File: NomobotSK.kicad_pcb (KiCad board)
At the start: 2 copper layers, 106.8 x 107.5 mm, 74 parts, among them J1 Conn_01x12_Pin, J2 Conn_01x03_Socket, J3 Conn_01x03_Socket, J4 Conn_01x03_Socket, J5 Conn_01x12_Pin, J6 Conn_01x12_Pin, M1 Motor_DC, M2 Motor_DC, SW1 SW_DIP_x01, SW2 SW_Push, SW3 SW_Push, SW4 SW_Push, SW5 SW_DIP_x10, SW6 SW_DIP_x04, U1 L293D, U2 TP4056 Module, U3 TCRT5000, U4 TCRT5000, U5 HC-SR04, U6 AMS1117-3.3, U7 LM393D

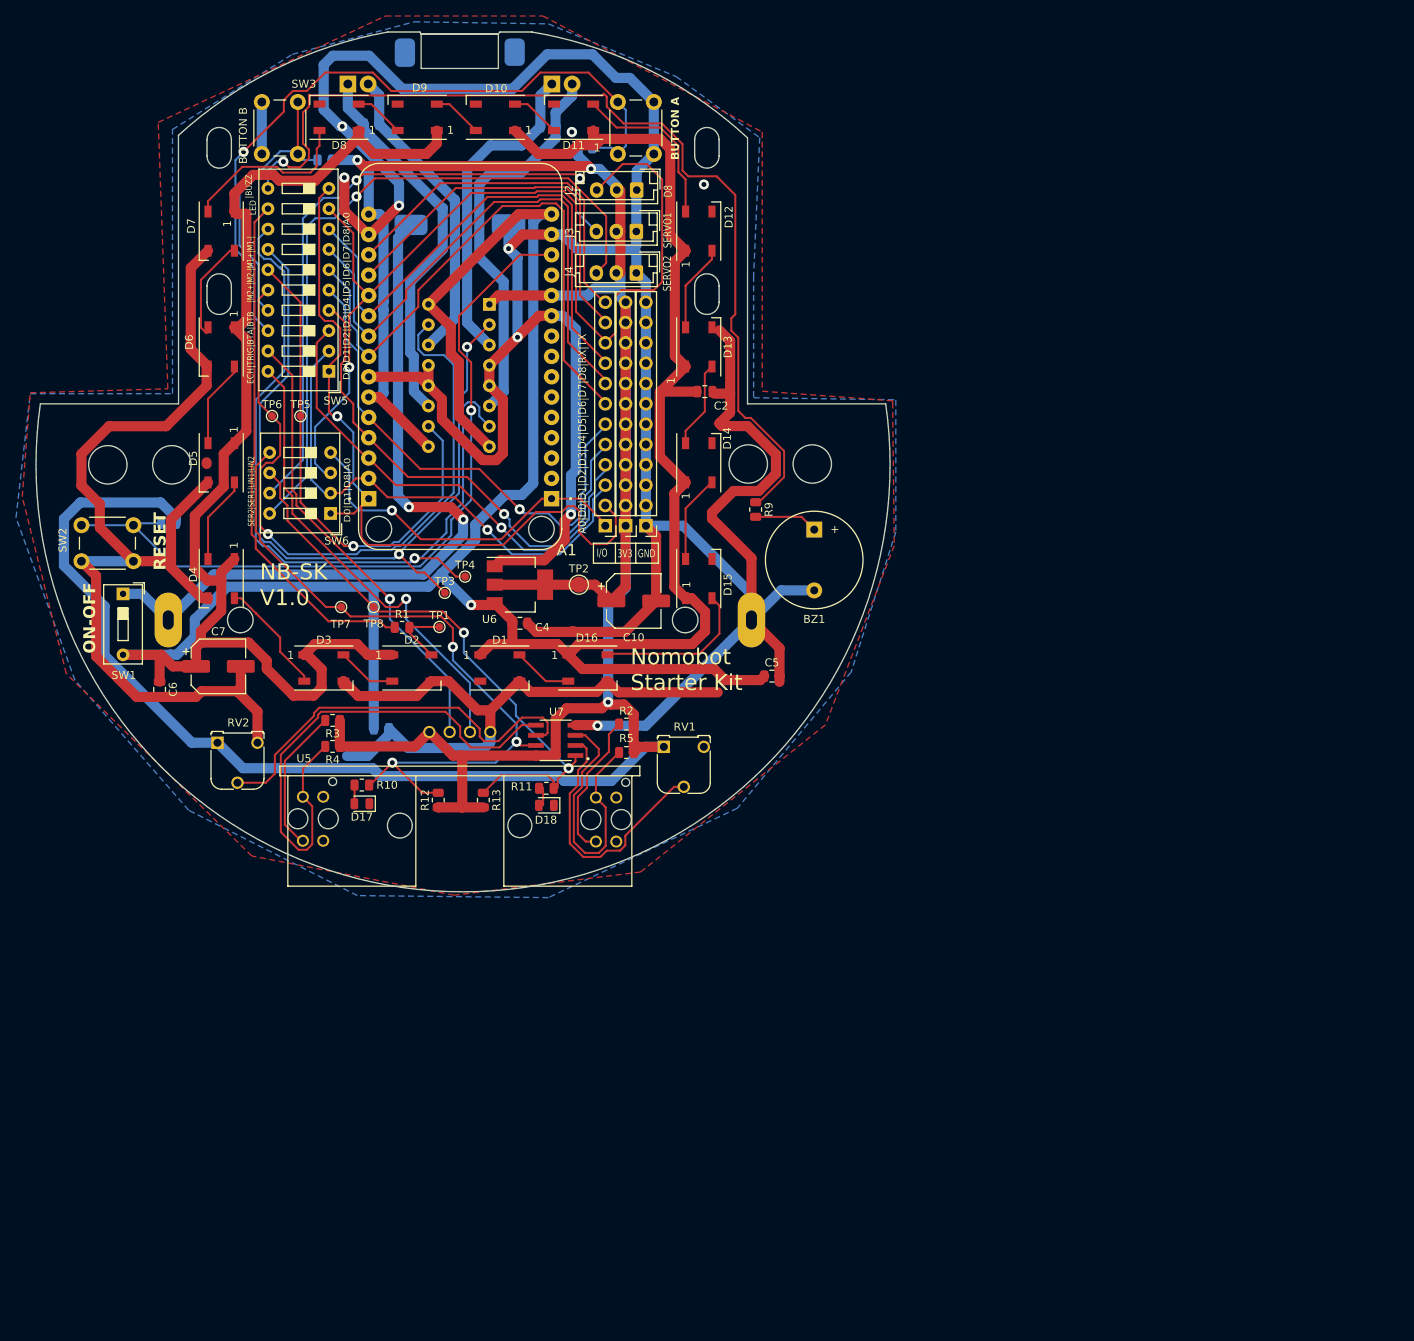
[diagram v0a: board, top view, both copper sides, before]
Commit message: routing done
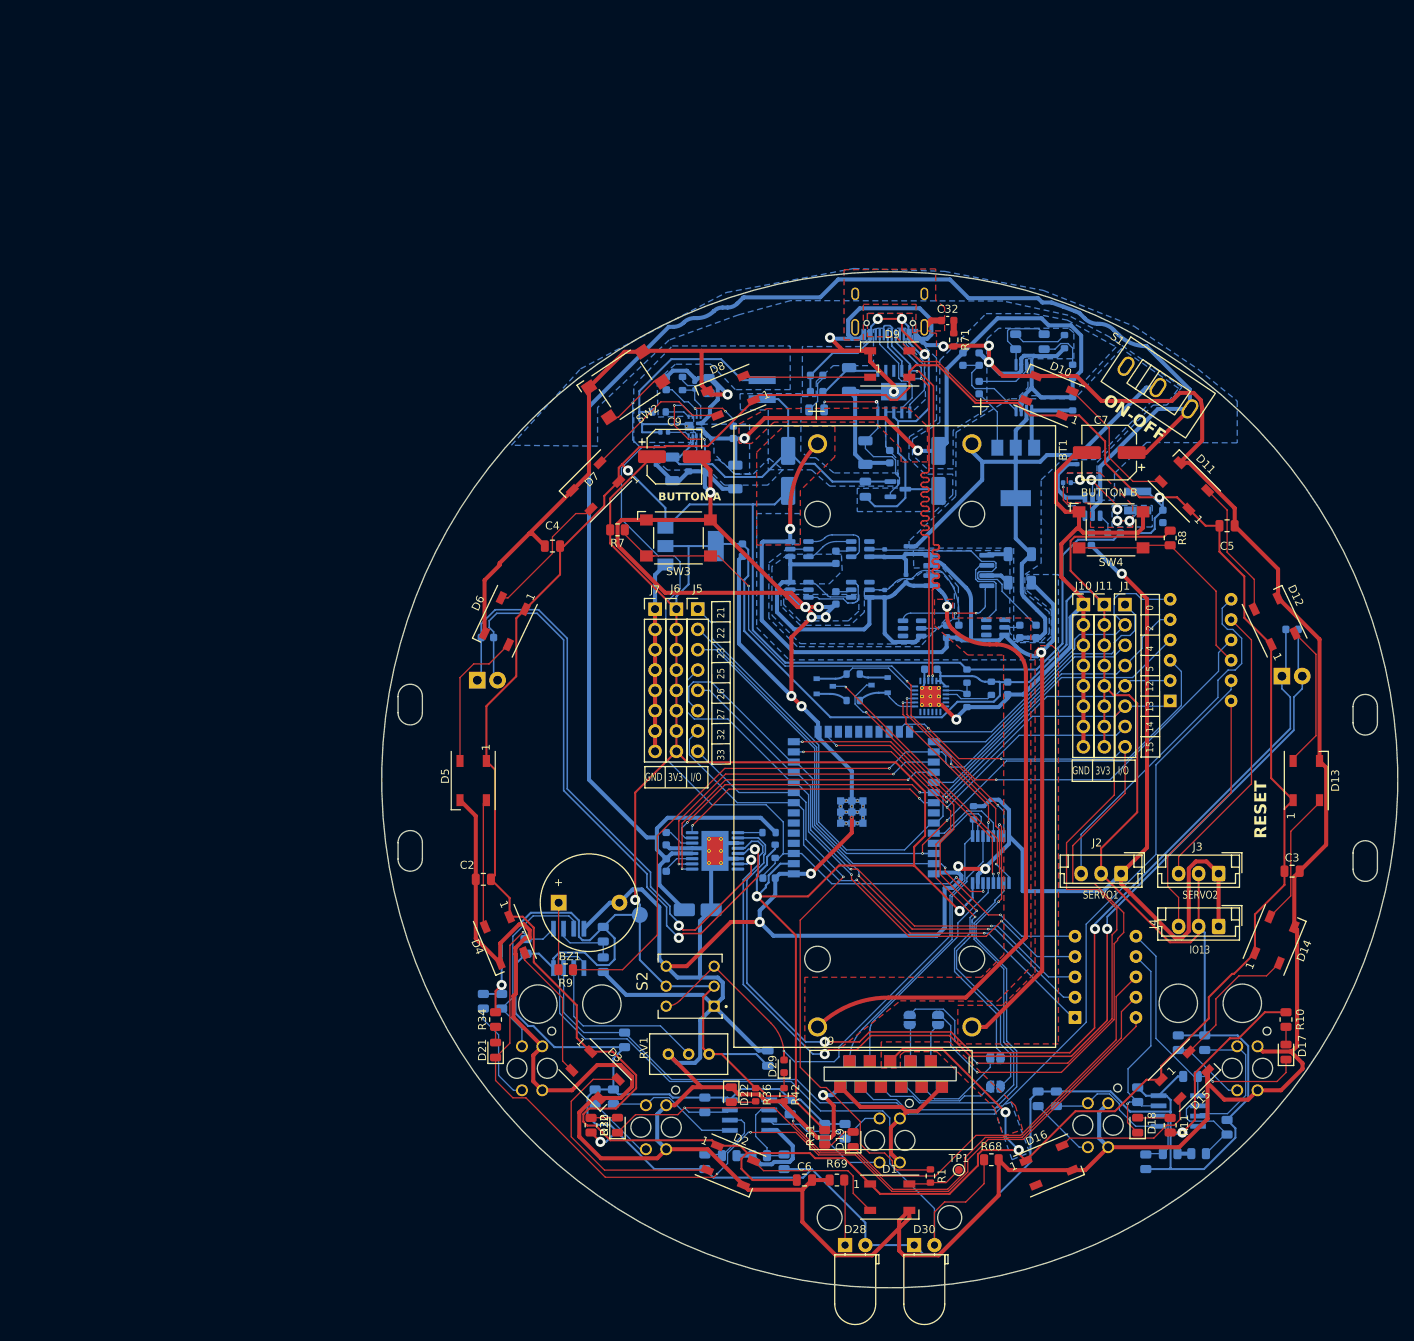
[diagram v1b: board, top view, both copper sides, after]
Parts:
- removed A1: NodeMCU V2 Amica, NodeMCU V2 AMICA:NodeMCU V2 Amica
- removed RV2: Trimpot_10K, Potentiometer_THT:Potentiometer_Runtron_RM-065_Vertical
- removed SW1: SW_DIP_x01, Button_Switch_THT:SW_DIP_SPSTx01_Slide_9.78x4.72mm_W7.62mm_P2.54mm
- removed TP3, TP4, TP5, TP6, TP7, TP8: TestPoint, TestPoint:TestPoint_Pad_D1.0mm
- added C11: 100nF, Capacitor_SMD:C_0603_1608Metric, B.Cu at (187.3, 112.3)
- added C12: 22uF/20V, Capacitor_SMD:C_0805_2012Metric, B.Cu at (190.5, 175.8)
- added C13: 4.7uF/6.3V, Capacitor_SMD:C_0603_1608Metric, B.Cu at (210.9, 127.2)
- added C14: 100nF/50V, Capacitor_SMD:C_0603_1608Metric, B.Cu at (220.5, 129.5)
- added C15: 100nF, Capacitor_SMD:C_0402_1005Metric, B.Cu at (177.5, 97.5)
- added C16: 47uF, Capacitor_SMD:C_1206_3216Metric, B.Cu at (186.4, 103.1)
- added C17: 47uF, Capacitor_SMD:C_1206_3216Metric, B.Cu at (178.6, 102.1)
- added C18: 100nF, Capacitor_SMD:C_0402_1005Metric, B.Cu at (176.5, 101.1)
- added C19: 10uF, Capacitor_SMD:C_0603_1608Metric, B.Cu at (182.6, 101.6)
- added C20: 470pF, Capacitor_SMD:C_0805_2012Metric, B.Cu at (183.1, 91.7)
- added C21: 24pF, Capacitor_SMD:C_0402_1005Metric, B.Cu at (181.4, 91.7)
- added C22: 100nF, Capacitor_SMD:C_0402_1005Metric, B.Cu at (207.8, 112.3)
- added C23: 100nF, Capacitor_SMD:C_0402_1005Metric, B.Cu at (207.8, 115.8)
- added C24: 100nF, Capacitor_SMD:C_0402_1005Metric, B.Cu at (205.1, 112.6)
- added C25: 100nF, Capacitor_SMD:C_0402_1005Metric, B.Cu at (205.1, 117.7)
- added C26: 1uF, Capacitor_SMD:C_1206_3216Metric, B.Cu at (200.7, 90.9)
- added C27: 1uF, Capacitor_SMD:C_1206_3216Metric, B.Cu at (202.7, 100.1)
- added C28: 100nF, Capacitor_SMD:C_0402_1005Metric, B.Cu at (229.2, 101.0)
- added C29: 10nF, Capacitor_SMD:C_0603_1608Metric, B.Cu at (177.8, 151.6)
- added C30: 100nF, Capacitor_SMD:C_0603_1608Metric, B.Cu at (256.0, 122.2)
- added C31: 100nF, Capacitor_SMD:C_0603_1608Metric, B.Cu at (155.4, 123.2)
- added C32: 100nF, Capacitor_SMD:C_0603_1608Metric, F.Cu at (213.0, 83.6)
- added C33: 100nF, Capacitor_SMD:C_0402_1005Metric, B.Cu at (227.9, 103.8)
- added C34: 22uF, Capacitor_SMD:C_0603_1608Metric, B.Cu at (239.9, 108.1)
- added C9: 22uF, Capacitor_SMD:CP_Elec_6.3x5.3, F.Cu at (178.8, 100.6)
- added D19: LED_Green, LED_SMD:LED_0805_2012Metric, F.Cu at (201.2, 185.9)
- added D20: LED_Green, LED_SMD:LED_0805_2012Metric, F.Cu at (171.7, 184.2)
- added D21: LED_Green, LED_SMD:LED_0805_2012Metric, F.Cu at (156.5, 174.8)
- added D22: LED_Blue, LED_SMD:LED_0805_2012Metric, F.Cu at (185.9, 180.3)
- added D23: LED_Red, LED_SMD:LED_0805_2012Metric, B.Cu at (221.5, 86.2)
- added D24: LED_Blue, LED_SMD:LED_0805_2012Metric, B.Cu at (196.6, 94.7)
- added D25: SS34, Diode_SMD:D_SMA_Handsoldering, B.Cu at (211.8, 102.4)
- added D26: SS34, Diode_SMD:D_SMA_Handsoldering, B.Cu at (193.0, 102.4)
- added D27: LED_Green, LED_SMD:LED_0805_2012Metric, B.Cu at (225.0, 86.2)
- added D28: IR_LED, LED_THT:LED_D5.0mm_Horizontal_O1.27mm_Z3.0mm_IRBlack, F.Cu at (200.2, 199.1)
- added D29: LED_RED, LED_SMD:LED_0603_1608Metric, F.Cu at (192.5, 176.8)
- added D30: IR_Photodiode, LED_THT:LED_D5.0mm_Horizontal_O1.27mm_Z3.0mm_Clear, F.Cu at (208.8, 199.1)
- added IC1: TS3A5018PW, TS3A5018PW:SOP65P640X120-16N, B.Cu at (218.4, 150.9)
- added J10: Conn_01x08_Pin, Connector_PinHeader_2.54mm:PinHeader_1x08_P2.54mm_Vertical, F.Cu at (229.9, 119.1)
- added J11: Conn_01x08_Pin, Connector_PinHeader_2.54mm:PinHeader_1x08_P2.54mm_Vertical, F.Cu at (232.6, 119.1)
- added J7: Conn_01x08_Pin, Connector_PinHeader_2.54mm:PinHeader_1x08_P2.54mm_Vertical, F.Cu at (176.4, 119.6)
- added J8: USB_C_Receptacle_USB2.0, Connector_USB:USB_C_Receptacle_HRO_TYPE-C-31-M-12, B.Cu at (205.7, 81.3)
- added J9: Conn_ESPCAM_Shield, Connector_Custom:Conn_ESPCAM_Shield-Female, F.Cu at (205.8, 178.7)
- added JP1: SolderJumper_2_Open, Jumper:SolderJumper-2_P1.3mm_Open_RoundedPad1.0x1.5mm, B.Cu at (218.9, 175.8)
- added JP2: SolderJumper_2_Open, Jumper:SolderJumper-2_P1.3mm_Open_RoundedPad1.0x1.5mm, B.Cu at (208.2, 171.0)
- added JP3: SolderJumper_2_Open, Jumper:SolderJumper-2_P1.3mm_Open_RoundedPad1.0x1.5mm, B.Cu at (211.8, 171.0)
- added JP4: SolderJumper_2_Open, Jumper:SolderJumper-2_P1.3mm_Open_RoundedPad1.0x1.5mm, B.Cu at (218.9, 179.3)
- added L1: XAL4020-102MEB_1uH, Inductor_SMD:L_Coilcraft_XAL4020-XXX, B.Cu at (189.8, 92.2)
- added L2: XAL4030-332MEB_3.3uH, Inductor_SMD:L_Coilcraft_XAL4030-XXX, B.Cu at (236.7, 106.1)
- added Q1: SS8050-G, SS8050-G:TRANS_SS8050-G, B.Cu at (204.5, 129.1)
- added Q2: SS8050-G, SS8050-G:TRANS_SS8050-G, B.Cu at (197.6, 129.3)
- added Q3: DMG9926UDM, Package_TO_SOT_SMD:SOT-23-6, B.Cu at (194.4, 112.1)
- added Q4: DMG9926UDM, Package_TO_SOT_SMD:SOT-23-6, B.Cu at (194.4, 117.2)
- added Q5: DMG9926USD-13, Package_SO:SO-8_5.3x6.2mm_P1.27mm, B.Cu at (214.4, 114.8)
- added Q6: AO3400A, Package_TO_SOT_SMD:SOT-23, B.Cu at (206.8, 104.6)
- added Q7: FZT788BTA, Package_TO_SOT_SMD:SOT-223-3_TabPin2, B.Cu at (221.5, 102.6)
- added R14: 220R, Resistor_SMD:R_0805_2012Metric, B.Cu at (197.6, 184.9)
- added R15: 220R, Resistor_SMD:R_0805_2012Metric, B.Cu at (168.9, 180.6)
- added R16: 10K, Resistor_SMD:R_0805_2012Metric, B.Cu at (200.2, 184.9)
- added R17: 10K, Resistor_SMD:R_0805_2012Metric, B.Cu at (171.2, 180.6)
- added R18: 220R, Resistor_SMD:R_0805_2012Metric, B.Cu at (154.9, 168.7)
- added R19: 10K, Resistor_SMD:R_0805_2012Metric, B.Cu at (157.2, 168.7)
- added R20: 10K, Resistor_SMD:R_0805_2012Metric, B.Cu at (240.8, 187.7)
- added R21: 10K, Resistor_SMD:R_0805_2012Metric, B.Cu at (237.7, 188.7)
- added R22: 10K, Resistor_SMD:R_0805_2012Metric, B.Cu at (247.9, 184.4)
- added R23: 10K, Resistor_SMD:R_0805_2012Metric, B.Cu at (244.3, 187.7)
- added R24: 10K, Resistor_SMD:R_0805_2012Metric, B.Cu at (192.5, 188.7)
- added R25: 10K, Resistor_SMD:R_0805_2012Metric, B.Cu at (182.6, 188.7)
- added R26: 10K, Resistor_SMD:R_0805_2012Metric, B.Cu at (185.7, 188.0)
- added R27: 10K, Resistor_SMD:R_0805_2012Metric, B.Cu at (189.5, 188.0)
- added R28: 10K, Resistor_SMD:R_0805_2012Metric, B.Cu at (182.6, 181.6)
- added R29: 10K, Resistor_SMD:R_0805_2012Metric, B.Cu at (193.3, 181.9)
- added R30: 10K, Resistor_SMD:R_0805_2012Metric, B.Cu at (169.9, 160.3)
- added R31: 470R, Resistor_SMD:R_0805_2012Metric, F.Cu at (197.6, 185.7)
- added R32: 470R, Resistor_SMD:R_0805_2012Metric, F.Cu at (168.4, 184.2)
- added R33: 10K, Resistor_SMD:R_0805_2012Metric, B.Cu at (169.9, 164.1)
- added R34: 470R, Resistor_SMD:R_0805_2012Metric, F.Cu at (156.5, 170.9)
- added R35: 10K, Resistor_SMD:R_0805_2012Metric, B.Cu at (160.3, 161.8)
- added R36: 220R, Resistor_SMD:R_0603_1608Metric, F.Cu at (189.0, 180.3)
- added R37: 28.7K, Resistor_SMD:R_0603_1608Metric, B.Cu at (179.8, 91.4)
- added R38: 10K, Resistor_SMD:R_0603_1608Metric, B.Cu at (201.2, 127.8)
- added R39: 10K, Resistor_SMD:R_0603_1608Metric, B.Cu at (201.2, 131.1)
- added R40: 10K, Resistor_SMD:R_0603_1608Metric, B.Cu at (218.4, 129.5)
- added R41: 10K, Resistor_SMD:R_0603_1608Metric, B.Cu at (216.2, 145.1)
- added R42: 330R, Resistor_SMD:R_0603_1608Metric, F.Cu at (192.5, 180.3)
- added R43: 22.1K, Resistor_SMD:R_0603_1608Metric, B.Cu at (215.4, 128.0)
- added R44: 47.5K, Resistor_SMD:R_0603_1608Metric, B.Cu at (215.4, 131.1)
- added R45: 649K, Capacitor_SMD:C_0603_1608Metric, B.Cu at (186.2, 97.5)
- added R46: 101K, Capacitor_SMD:C_0603_1608Metric, B.Cu at (177.8, 91.4)
- added R47: 100K, Resistor_SMD:R_0603_1608Metric, B.Cu at (176.9, 95.0)
- added R48: 107K, Resistor_SMD:R_0603_1608Metric, B.Cu at (180.6, 101.6)
- added R49: 1K, Resistor_SMD:R_1206_3216Metric, B.Cu at (222.0, 112.8)
- added R50: 1K, Resistor_SMD:R_1206_3216Metric, B.Cu at (222.0, 116.3)
- added R51: 100R, Capacitor_SMD:C_0603_1608Metric, B.Cu at (222.0, 122.4)
- added R52: 100R, Capacitor_SMD:C_0603_1608Metric, B.Cu at (212.9, 122.4)
- added R53: 100R, Capacitor_SMD:C_0603_1608Metric, B.Cu at (224.0, 122.4)
- added R54: 1K, Capacitor_SMD:C_0603_1608Metric, B.Cu at (199.0, 113.2)
- added R55: 1K, Capacitor_SMD:C_0603_1608Metric, B.Cu at (199.0, 118.2)
- added R56: 100R, Capacitor_SMD:C_0603_1608Metric, B.Cu at (214.4, 122.4)
- added R57: 6.8K, Capacitor_SMD:C_0603_1608Metric, B.Cu at (205.7, 100.6)
- added R58: 1K, Capacitor_SMD:C_0603_1608Metric, B.Cu at (196.6, 92.5)
- added R59: 1K, Capacitor_SMD:C_0603_1608Metric, B.Cu at (196.6, 90.4)
- added R60: 0R, Capacitor_SMD:C_0805_2012Metric, B.Cu at (202.7, 104.6)
- added R61: 1K, Capacitor_SMD:C_0603_1608Metric, B.Cu at (216.9, 91.9)
- added R62: 280R, Resistor_SMD:R_0603_1608Metric, B.Cu at (227.6, 86.2)
- added R63: 280R, Resistor_SMD:R_0603_1608Metric, B.Cu at (228.6, 89.9)
- added R64: 0.2R, Resistor_SMD:R_0603_1608Metric, B.Cu at (228.6, 94.0)
- added R65: 1K, Capacitor_SMD:C_0603_1608Metric, B.Cu at (214.9, 88.4)
- added R66: 1K, Capacitor_SMD:C_0603_1608Metric, B.Cu at (216.9, 88.4)
- added R67: 47K, Resistor_SMD:R_0603_1608Metric, B.Cu at (190.7, 147.6)
- added R68: 10K, Resistor_SMD:R_0805_2012Metric, F.Cu at (218.4, 188.5)
- added R69: 220R, Resistor_SMD:R_0805_2012Metric, F.Cu at (199.1, 191.0)
- added R70: 10K, Resistor_SMD:R_0805_2012Metric, B.Cu at (172.6, 173.5)
- added R71: 220R, Resistor_SMD:R_0603_1608Metric, F.Cu at (213.7, 86.0)
- added R72: 10K, Capacitor_SMD:C_0603_1608Metric, B.Cu at (230.9, 110.9)
- added R73: 56.2K, Capacitor_SMD:C_0603_1608Metric, B.Cu at (233.8, 110.1)
- added S1: SW_SS12D10, Switch Custom:SW_SS-12D10-G5050, F.Cu at (239.3, 91.9)
- added S2: SW_DPDT_TL2285EE, Switch Custom:SW_TL2285EE, F.Cu at (180.8, 166.8)
- added U10: TCRT5000, TCRT5000:OPTO_TCRT5000, B.Cu at (161.0, 177.0)
- added U11: LM393D, LM393D:SOIC127P599X175-8N, B.Cu at (188.2, 182.9)
- added U12: LM393D, LM393D:SOIC127P599X175-8N, B.Cu at (165.6, 162.1)
- added U13: ESP32-WROOM-32E__16MB_, ESP32-WROOM-32E:XCVR_ESP32-WROOM-32E__16MB_, B.Cu at (202.5, 147.5)
- added U14: CP2102N-Axx-xQFN24, Package_DFN_QFN:QFN-24-1EP_4x4mm_P0.5mm_EP2.6x2.6mm_ThermalVias, B.Cu at (210.8, 130.6)
- added U15: DW01A, Package_TO_SOT_SMD:SOT-23-6, B.Cu at (202.1, 112.1)
- added U16: DW01A, Package_TO_SOT_SMD:SOT-23-6, B.Cu at (202.1, 117.2)
- added U17: HY2213-BB3A, Package_TO_SOT_SMD:SOT-23-6, B.Cu at (218.9, 121.9)
- added U18: HY2213-BB3A, Package_TO_SOT_SMD:SOT-23-6, B.Cu at (208.5, 122.0)
- added U19: CH224K, CH224K:ESSOP-10, B.Cu at (206.2, 92.5)
- added U21: BQ2057WTSTR, Package_SO:TSSOP-8_4.4x3mm_P0.65mm, B.Cu at (222.5, 91.9)
- added U8: TCRT5000, TCRT5000:OPTO_TCRT5000, B.Cu at (205.7, 186.1)
- added U9: TCRT5000, TCRT5000:OPTO_TCRT5000, B.Cu at (176.5, 184.4)
- BT1: value BH-18650-PC -> BK-18650-PC4; footprint BH-18650-PC:BAT_BH-18650-PC -> BK-18650-PC4:BAT_BK-18650-PC4; moved to F.Cu
- C1: value 1u -> 10uF/16V; footprint Capacitor_SMD:C_0805_2012Metric -> Capacitor_SMD:C_Elec_4x5.4
- C10: value C_Polarized -> 100nF; footprint Capacitor_SMD:CP_Elec_6.3x5.3 -> Capacitor_SMD:C_0603_1608Metric; moved to B.Cu
- C2, C4, C5, C6: value 100n -> 100nF
- C3: value 100n -> 100nF; moved to F.Cu
- C7: value C_Polarized -> 10uF
- C8: value 1u -> 2.2uF; footprint Capacitor_SMD:C_0805_2012Metric -> Capacitor_SMD:C_0603_1608Metric
- J1, J5, J6: value Conn_01x12_Pin -> Conn_01x08_Pin; footprint Connector_PinHeader_2.54mm:PinHeader_1x12_P2.54mm_Vertical -> Connector_PinHeader_2.54mm:PinHeader_1x08_P2.54mm_Vertical
- R1, R6: footprint Resistor_SMD:R_0805_2012Metric -> Resistor_SMD:R_0603_1608Metric
- R10, R11: value 330R -> 470R
- R12, R13: value 1K -> 10K; moved to B.Cu
- R2, R3, R4, R5, TP2, U6, U7: moved to B.Cu
- R7, R8: moved to F.Cu
- RV1: value Trimpot_10K -> R_Potentiometer_10K; footprint Potentiometer_THT:Potentiometer_Runtron_RM-065_Vertical -> Potentiometer_THT:Potentiometer_Bourns_3296W_Vertical
- SW2, SW3, SW4: value SW_Push -> SW_SPST_Omron_B3FS-105xP; footprint Button_Switch_THT:SW_PUSH_6mm_H4.3mm -> Button_Switch_SMD:SW_SPST_Omron_B3FS-105xP
- SW5: value SW_DIP_x10 -> SW_DIP_x06; footprint Button_Switch_THT:SW_DIP_SPSTx10_Slide_9.78x27.58mm_W7.62mm_P2.54mm -> Button_Switch_THT:SW_DIP_SPSTx06_Slide_9.78x17.42mm_W7.62mm_P2.54mm; moved to B.Cu
- SW6: value SW_DIP_x04 -> SW_DIP_x05; footprint Button_Switch_THT:SW_DIP_SPSTx04_Slide_9.78x12.34mm_W7.62mm_P2.54mm -> Button_Switch_THT:SW_DIP_SPSTx05_Slide_9.78x14.88mm_W7.62mm_P2.54mm; moved to B.Cu
- U1: value L293D -> DRV8833PWP; footprint Package_DIP:DIP-16_W7.62mm -> Package_SO:HTSSOP-16-1EP_4.4x5mm_P0.65mm_EP3.4x5mm_Mask2.46x2.31mm_ThermalVias
- U2: value TP4056 Module -> TPS61089RNRR; footprint Modules:TP4056_Module -> TPS61089RNRR:IC_TPS61089RNRR
- U5: value HC-SR04 -> TPS563201; footprint HC-SR04:XCVR_HC-SR04 -> Package_TO_SOT_SMD:SOT-23-6; moved to B.Cu
- moved D17 119.6 mm to (255.3, 175.0), turned to 90 degrees
- moved R10 119.2 mm to (255.3, 170.9), turned to 90 degrees
- moved M1 117.5 mm to (254.8, 128.0)
- moved R8 115.7 mm to (240.8, 110.7), turned to 90 degrees
- moved C3 115.2 mm to (256.0, 152.4)
- moved C7 114.5 mm to (233.2, 100.1), turned to 180 degrees
- moved SW5 112.9 mm to (240.8, 131.1), turned to 0 degrees
- moved SW6 112.4 mm to (228.9, 170.7), turned to 0 degrees
- moved J4 109.4 mm to (246.8, 159.3)
- moved J3 108.4 mm to (246.8, 152.7)
- moved C1 106.3 mm to (181.7, 157.2)
- moved U4 105.3 mm to (231.8, 184.2)
- moved J2 104.7 mm to (234.7, 152.7)
- moved C6 101.3 mm to (195.1, 191.0), turned to 0 degrees
- moved R4 100.6 mm to (226.6, 180.8), turned to -90 degrees
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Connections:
- net SIG_L renamed /LINE SENSOR/SIG_1
- net SIG_R renamed /LINE SENSOR/SIG_2
- C1 pad 1: M2P -> /POWER/VBAT
- C1 pad 2: M2N -> GND
- C10 pad 1: 3V3 -> GND
- C10 pad 2: GND -> /MAIN MCU/EN
- C2 pad 1: VBAT+ -> /VCC
- C3 pad 1: VBAT+ -> /VCC
- C4 pad 1: VBAT+ -> /VCC
- C5 pad 1: VBAT+ -> /VCC
- C6 pad 1: VBAT+ -> /VCC
- C7 pad 1: VBAT+ -> /POWER/VBAT
- C8 pad 1: M1P -> Net-(U1-VINT)
- C8 pad 2: M1N -> GND
- D1 pad 1: VBAT+ -> /VCC
- D1 pad 2: unconnected-(D1-DOUT-Pad2) -> Net-(D1-DOUT)
- D1 pad 4: Net-(D1-DIN) -> /MAIN MCU/LED_DIN
- D10 pad 1: VBAT+ -> /VCC
- D11 pad 1: VBAT+ -> /VCC
- D12 pad 1: VBAT+ -> /VCC
- D13 pad 1: VBAT+ -> /VCC
- D14 pad 1: VBAT+ -> /VCC
- D15 pad 1: VBAT+ -> /VCC
- D16 pad 1: VBAT+ -> /VCC
- D16 pad 2: Net-(D1-DIN) -> unconnected-(D16-DOUT-Pad2)
- D17 pad 1: GND -> /LINE SENSOR/LIN_1
- D18 pad 1: GND -> /LINE SENSOR/LIN_2
- D2 pad 1: VBAT+ -> /VCC
- D2 pad 4: LED_DIN -> Net-(D1-DOUT)
- D3 pad 1: VBAT+ -> /VCC
- D4 pad 1: VBAT+ -> /VCC
- D5 pad 1: VBAT+ -> /VCC
- D6 pad 1: VBAT+ -> /VCC
- D7 pad 1: VBAT+ -> /VCC
- D8 pad 1: VBAT+ -> /VCC
- D9 pad 1: VBAT+ -> /VCC
- J1 pad 1: A0 -> /MAIN MCU/IO0
- J1 pad 2: D0 -> /MAIN MCU/IO2
- J1 pad 3: D1 -> /MAIN MCU/IO4
- J1 pad 4: D2 -> /MAIN MCU/IO5
- J1 pad 5: D3 -> /MAIN MCU/IO12
- J1 pad 6: D4 -> /MAIN MCU/IO13
- J1 pad 7: D5 -> /MAIN MCU/IO14
- J1 pad 8: D6 -> /MAIN MCU/IO15
- J2 pad 2: 3V3 -> /VDD
- J2 pad 3: D8 -> /MAIN MCU/SERVO_R
- J3 pad 2: 3V3 -> /VDD
- J3 pad 3: SERVO_R -> /MAIN MCU/SERVO_L
- J4 pad 2: 3V3 -> /VDD
- J4 pad 3: SERVO_L -> /MAIN MCU/I/O Pin
- J5 pad 1: 3V3 -> /MAIN MCU/IO21
- J5 pad 2: 3V3 -> /MAIN MCU/IO22
- J5 pad 3: 3V3 -> /MAIN MCU/IO23
- J5 pad 4: 3V3 -> /MAIN MCU/IO25
- J5 pad 5: 3V3 -> /MAIN MCU/IO26
- J5 pad 6: 3V3 -> /MAIN MCU/IO27
- J5 pad 7: 3V3 -> /MAIN MCU/IO32
- J5 pad 8: 3V3 -> /MAIN MCU/IO33
- J6 pad 1: GND -> /VDD
- J6 pad 2: GND -> /VDD
- J6 pad 3: GND -> /VDD
- J6 pad 4: GND -> /VDD
- J6 pad 5: GND -> /VDD
- J6 pad 6: GND -> /VDD
- J6 pad 7: GND -> /VDD
- J6 pad 8: GND -> /VDD
- R1 pad 1: Net-(R1-Pad1) -> /MAIN MCU/IO33
- R1 pad 2: LED_DIN -> /MAIN MCU/LED_DIN
- R10 pad 1: LIN_R -> Net-(D17-A)
- R10 pad 2: Net-(D17-A) -> /VDD
- R11 pad 1: LIN_L -> Net-(D18-A)
- R11 pad 2: Net-(D18-A) -> /VDD
- R12 pad 1: 3V3 -> /VDD
- R12 pad 2: LIN_R -> /LINE SENSOR/LIN_2
- R13 pad 1: LIN_L -> /LINE SENSOR/LIN_1
- R13 pad 2: 3V3 -> /VDD
- R2 pad 2: 3V3 -> /VDD
- R3 pad 1: 3V3 -> Net-(R3-Pad1)
- R3 pad 2: Net-(R3-Pad2) -> /VDD
- R4 pad 1: 3V3 -> /VDD
- R5 pad 1: 3V3 -> /VDD
- R6 pad 1: Button2 -> /MAIN MCU/EN
- R6 pad 2: 3V3 -> /VDD
- R7 pad 1: 3V3 -> /MAIN MCU/Button1
- R7 pad 2: reset -> /VDD
- R8 pad 1: Button1 -> /MAIN MCU/Button2
- R8 pad 2: 3V3 -> /VDD
- R9 pad 1: BUZZ -> /MAIN MCU/IO4
- RV1 pad 1: 3V3 -> /VDD
- RV1 pad 2: Net-(U7-1IN-) -> /LINE SENSOR/PROX_COMP
- SW2 pad 2: reset -> /MAIN MCU/EN
- SW3 pad 2: Button1 -> /MAIN MCU/Button1
- SW4 pad 2: Button2 -> /MAIN MCU/Button2
- SW5 pad 1: D0 -> /MAIN MCU/IO13
- SW5 pad 10: D0 -> /MAIN MCU/Button2
- SW5 pad 11: BUZZ -> /LINE SENSOR/PROX_OUT
- SW5 pad 12: Net-(R1-Pad1) -> /MAIN MCU/I/O Pin
- SW5 pad 2: D1 -> /MAIN MCU/IO12
- SW5 pad 3: D2 -> /MAIN MCU/IO22
- SW5 pad 4: D3 -> /MAIN MCU/IO21
- SW5 pad 5: D4 -> /MAIN MCU/IO5
- SW5 pad 6: D5 -> /MAIN MCU/IO2
- SW5 pad 7: D6 -> /MAIN MCU/SERVO_R
- SW5 pad 8: D7 -> /MAIN MCU/SERVO_L
- SW5 pad 9: D8 -> /MAIN MCU/Button1
- SW6 pad 1: D0 -> /MAIN MCU/IO32
- SW6 pad 2: D1 -> /MAIN MCU/IO27
- SW6 pad 3: D8 -> /MAIN MCU/IO26
- SW6 pad 4: A0 -> /MAIN MCU/IO25
- SW6 pad 5: LIN_R -> /MAIN MCU/IO23
- SW6 pad 6: LIN_L -> /LINE SENSOR/LIN_1
- SW6 pad 7: SERVO_R -> /LINE SENSOR/LIN_2
- SW6 pad 8: SERVO_L -> /LINE SENSOR/LIN_3
- TP1 pad 1: LED_DIN -> /MAIN MCU/LED_DIN
- TP2 pad 1: 3V3 -> /VDD
- U1 pad 1: 3V3 -> Net-(U1-nSLEEP)
- U1 pad 10: DIR2_R -> /MAIN MCU/IO16
- U1 pad 11: M2P -> Net-(U1-VCP)
- U1 pad 12: GND -> /POWER/VBAT
- U1 pad 14: M2N -> Net-(U1-VINT)
- U1 pad 15: DIR2_F -> /MAIN MCU/IO18
- U1 pad 16: VBAT+ -> /MAIN MCU/IO19
- U1 pad 2: DIR1_F -> M1P
- U1 pad 3: M1P -> GND
- U1 pad 4: GND -> M1N
- U1 pad 5: GND -> M2N
- U1 pad 6: M1N -> GND
- U1 pad 7: DIR1_R -> M2P
- U1 pad 8: VBAT+ -> unconnected-(U1-nFAULT-Pad8)
- U1 pad 9: 3V3 -> /MAIN MCU/IO17
- U2 pad 1: unconnected-(U2-USB+-Pad1) -> Net-(U2-FSW)
- U2 pad 2: unconnected-(U2-USB--Pad2) -> /POWER/VCC_U2
- U2 pad 3: VBAT -> Net-(U2-FB)
- U2 pad 4: GND -> Net-(U2-COMP)
- U4 pad A: Net-(R3-Pad2) -> Net-(R3-Pad1)
- U5 pad 1: 3V3 -> GND
- U5 pad 2: TRIG -> /POWER/LPADbuck
- U5 pad 3: ECHO -> /POWER/VBAT
- U5 pad 4: GND -> Net-(U5-VFB)
- U6 pad 2: 3V3 -> /VDD
- U6 pad 3: VBAT+ -> /VCC
- U7 pad 1: LIN_L -> /LINE SENSOR/LIN_1
- U7 pad 7: LIN_R -> /LINE SENSOR/LIN_2
- U7 pad 8: 3V3 -> /VDD
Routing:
- net /VDD: track 0.00 -> 747.3 mm, vias 0 -> 6
- net GND: track 615.0 -> 1174.5 mm, vias 9 -> 20
- net /VCC: track 0.00 -> 512.1 mm, vias 0 -> 4
- net VBAT+: track 477.8 -> 0.00 mm, vias 1 -> 0
- net 3V3: track 404.6 -> 0.00 mm, vias 3 -> 0
- net /POWER/VBAT: track 0.00 -> 208.9 mm
- net /POWER/BAT_MID: track 0.00 -> 152.0 mm, vias 0 -> 2
- net /MAIN MCU/IO13: track 0.00 -> 131.5 mm, vias 0 -> 3
- net /LINE SENSOR/PROX_OUT: track 0.00 -> 131.1 mm
- net /POWER/BAT-: track 0.00 -> 131.0 mm, vias 0 -> 1
- net /LINE SENSOR/LIN_5: track 0.00 -> 126.7 mm, vias 0 -> 3
- net D8: track 126.2 -> 0.00 mm, vias 1 -> 0
- net BUZZ: track 121.9 -> 0.00 mm, vias 1 -> 0
- net /MAIN MCU/EN: track 0.00 -> 114.4 mm, vias 0 -> 3
- net /MAIN MCU/Button1: track 0.00 -> 103.1 mm, vias 0 -> 3
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- added copper zone on B.Cu, net /CONNECTOR/VBUS
- added copper zone on F.Cu, net /CONNECTOR/VBUS
- added copper zone on B.Cu, net /POWER/9V
- added copper zone on F.Cu, net /POWER/9V
- added copper zone on B.Cu, net /POWER/BAT+
- added copper zone on B.Cu, net /POWER/BAT-
- added copper zone on F.Cu, net /POWER/BAT-
- added copper zone on B.Cu, net /POWER/BAT_MID
- added copper zone on F.Cu, net /POWER/BAT_MID
- added copper zone on B.Cu, net /POWER/LPADbuck
- added copper zone on F.Cu, net /POWER/LPADbuck
- added copper zone on B.Cu, net /POWER/PadL
- added copper zone on B.Cu, net /POWER/VBAT
- added copper zone on B.Cu, net /POWER/VIN_U2
- added copper zone on B.Cu, net /VCC
- added copper zone on F.Cu, net /VCC
- added copper zone on F.Cu, net Net-(J8-SHIELD)
- removed copper zone on F.Cu, net GND
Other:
- board size 106.8 x 107.5 mm -> 127 x 127 mm
- board text added: "0"
- board text added: "12"
- board text added: "13"
- board text added: "14"
- board text added: "15"
- board text added: "2"
- board text added: "21"
- board text added: "22"
- board text added: "23"
- board text added: "25"
- board text added: "26"
- board text added: "27"
- board text added: "32"
- board text added: "33"
- board text added: "4"
- board text added: "5"
- board text added: "IO13"
- board text removed: "A0|D0|D1|D2|D3|D4|D5|D6|D7|D8|RX|TX"
- board text removed: "D0|D1|D2|D3|D4|D5|D6|D7|D8|A0"
- board text removed: "D0|D1|D8|A0"
- board text removed: "D8"
- board text removed: "ECH|TRIG|BTA|BTB"
- board text removed: "LED"
- board text removed: "NB-SK V1.0"
- board text removed: "Nomobot Starter Kit"
- board text removed: "SER2|SER1|LIN1|LIN2"
- board text removed: "|BUZZ"
- board text removed: "|M2+|M2-|M1+|M1-|"
